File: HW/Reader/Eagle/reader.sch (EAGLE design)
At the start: 47 parts, among them Q4 BC817, U1 MCP16311, U2 ESP8266-12E

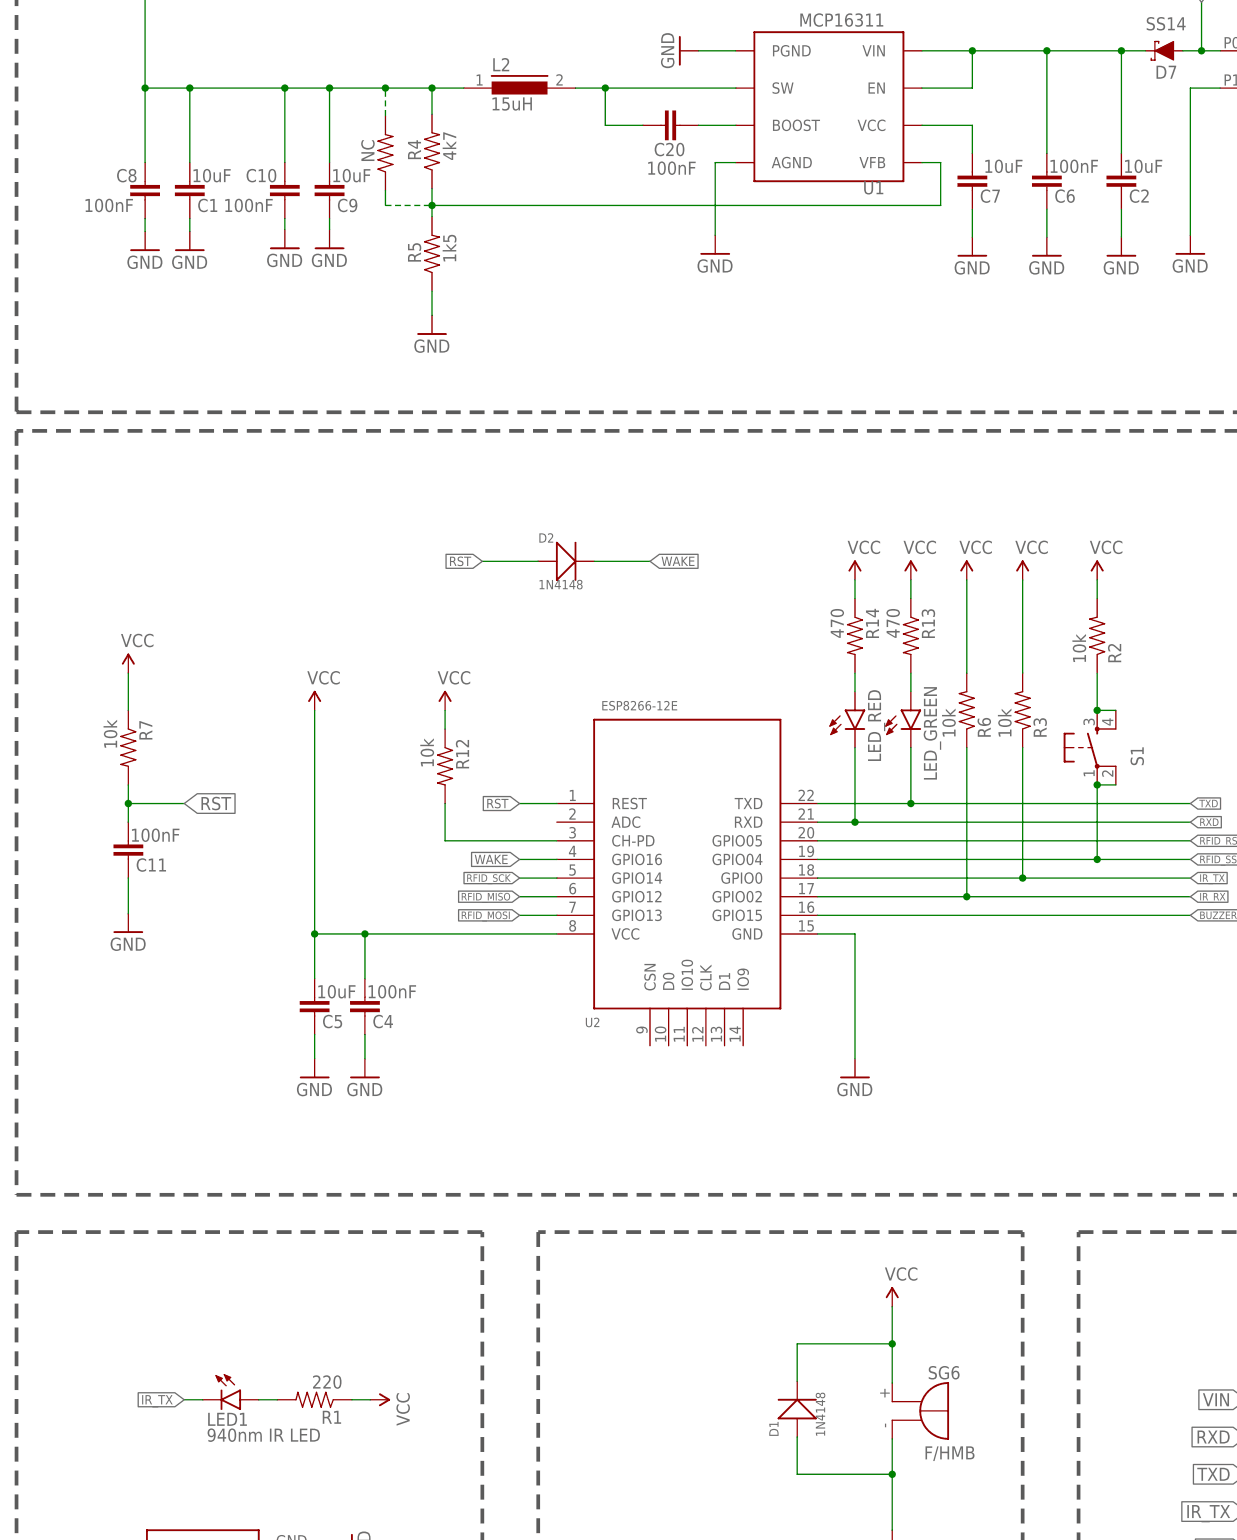
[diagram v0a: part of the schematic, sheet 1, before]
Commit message: Schematics are updated
Kickstart flasher PCB
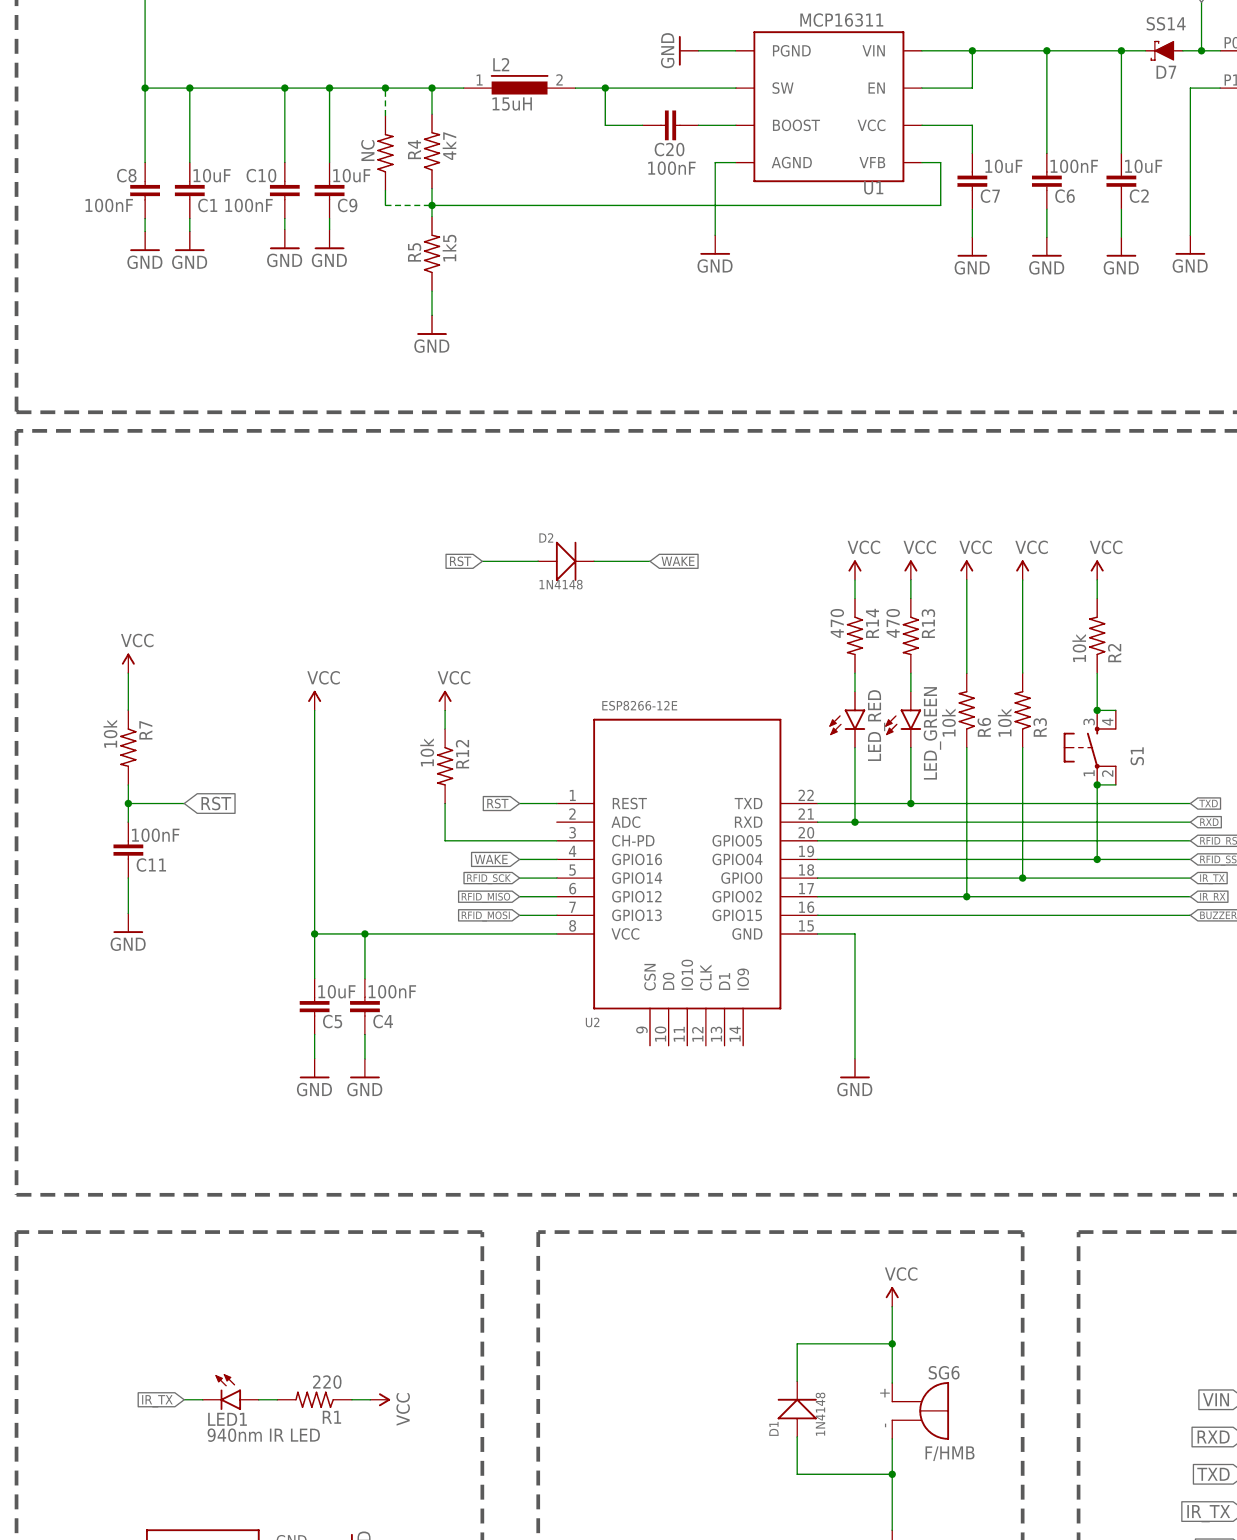
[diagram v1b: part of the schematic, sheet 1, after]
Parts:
- NC, R1, R12, R13, R14, R2, R3, R4, R5, R6, R7: device antduino:SPARKFUN_RESISTOR0805-RES -> rcl:R-US_M0805
- R10, R11: device adafruit:R-US_M0805 -> rcl:R-US_M0805
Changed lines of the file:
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@@
 <?xml version="1.0" encoding="utf-8"?>
 <!DOCTYPE eagle SYSTEM "eagle.dtd">
-<eagle version="9.6.0">
+<eagle version="9.6.1">
 <drawing>
 <settings>
@@
 <part name="GND17" library="supply1" deviceset="GND" device=""/>
 <part name="C12" library="rcl" library_urn="urn:adsk.eagle:library:334" deviceset="C-EU" device="C0805" package3d_urn="urn:adsk.eagle:package:23617/2" value="10uF"/>
-<part name="R1" library="antduino" deviceset="SPARKFUN_RESISTOR" device="0805-RES" value="220"/>
+<part name="R1" library="rcl" library_urn="urn:adsk.eagle:library:334" deviceset="R-US_" device="M0805" package3d_urn="urn:adsk.eagle:package:23556/2" value="220"/>
 <part name="GND3" library="supply1" library_urn="urn:adsk.eagle:library:371" deviceset="GND" device=""/>
 <part name="GND4" library="supply1" library_urn="urn:adsk.eagle:library:371" deviceset="GND" device=""/>
@@
 <part name="SUPPLY4" library="SparkFun-Aesthetics" deviceset="VCC" device=""/>
 <part name="Q4" library="dp_devices" deviceset="TRANSISTOR_BJT_NPN" device="-SOT-23-BCE" value="BC817"/>
-<part name="R10" library="adafruit" deviceset="R-US_" device="M0805" value="4k7"/>
-<part name="R11" library="adafruit" deviceset="R-US_" device="M0805" value="1K"/>
+<part name="R10" library="rcl" library_urn="urn:adsk.eagle:library:334" deviceset="R-US_" device="M0805" package3d_urn="urn:adsk.eagle:package:23556/2" value="4k7"/>
+<part name="R11" library="rcl" library_urn="urn:adsk.eagle:library:334" deviceset="R-US_" device="M0805" package3d_urn="urn:adsk.eagle:package:23556/2" value="1K"/>
 <part name="SUPPLY5" library="SparkFun-Aesthetics" deviceset="VCC" device=""/>
 <part name="SUPPLY6" library="SparkFun-Aesthetics" deviceset="VCC" device=""/>
@@
 <part name="GND18" library="supply1" deviceset="GND" device=""/>
 <part name="GND19" library="supply1" deviceset="GND" device=""/>
-<part name="R4" library="antduino" deviceset="SPARKFUN_RESISTOR" device="0805-RES" value="4k7"/>
-<part name="R5" library="antduino" deviceset="SPARKFUN_RESISTOR" device="0805-RES" value="1k5"/>
+<part name="R4" library="rcl" library_urn="urn:adsk.eagle:library:334" deviceset="R-US_" device="M0805" package3d_urn="urn:adsk.eagle:package:23556/2" value="4k7"/>
+<part name="R5" library="rcl" library_urn="urn:adsk.eagle:library:334" deviceset="R-US_" device="M0805" package3d_urn="urn:adsk.eagle:package:23556/2" value="1k5"/>
 <part name="GND20" library="supply1" deviceset="GND" device=""/>
-<part name="NC" library="antduino" deviceset="SPARKFUN_RESISTOR" device="0805-RES"/>
+<part name="NC" library="rcl" library_urn="urn:adsk.eagle:library:334" deviceset="R-US_" device="M0805" package3d_urn="urn:adsk.eagle:package:23556/2"/>
 <part name="SUPPLY7" library="SparkFun-Aesthetics" deviceset="VCC" device=""/>
 <part name="GND21" library="supply1" deviceset="GND" device=""/>
@@
 <part name="GND25" library="supply1" deviceset="GND" device=""/>
 <part name="M2" library="mfrc522-module" deviceset="RFID-RC522" device=""/>
-<part name="R12" library="antduino" deviceset="SPARKFUN_RESISTOR" device="0805-RES" value="10k"/>
+<part name="R12" library="rcl" library_urn="urn:adsk.eagle:library:334" deviceset="R-US_" device="M0805" package3d_urn="urn:adsk.eagle:package:23556/2" value="10k"/>
 <part name="SUPPLY3" library="SparkFun-Aesthetics" deviceset="VCC" device=""/>
 <part name="READER" library="frames" library_urn="urn:adsk.eagle:library:229" deviceset="FRAME_B_L" device=""/>
-<part name="R13" library="antduino" deviceset="SPARKFUN_RESISTOR" device="0805-RES" value="470"/>
-<part name="R14" library="antduino" deviceset="SPARKFUN_RESISTOR" device="0805-RES" value="470"/>
+<part name="R13" library="rcl" library_urn="urn:adsk.eagle:library:334" deviceset="R-US_" device="M0805" package3d_urn="urn:adsk.eagle:package:23556/2" value="470"/>
+<part name="R14" library="rcl" library_urn="urn:adsk.eagle:library:334" deviceset="R-US_" device="M0805" package3d_urn="urn:adsk.eagle:package:23556/2" value="470"/>
 <part name="SUPPLY9" library="SparkFun-Aesthetics" deviceset="VCC" device=""/>
 <part name="SUPPLY10" library="SparkFun-Aesthetics" deviceset="VCC" device=""/>
@@
 <part name="S1" library="SparkFun" deviceset="TAC_SWITCH" device="PTH" value="FLASH"/>
 <part name="U$1" library="Terminal Block Connector" deviceset="DBCONN-1X2" device=""/>
-<part name="R2" library="antduino" deviceset="SPARKFUN_RESISTOR" device="0805-RES" value="10k"/>
+<part name="R2" library="rcl" library_urn="urn:adsk.eagle:library:334" deviceset="R-US_" device="M0805" package3d_urn="urn:adsk.eagle:package:23556/2" value="10k"/>
 <part name="SUPPLY8" library="SparkFun-Aesthetics" deviceset="VCC" device=""/>
 <part name="TP1" library="testpad" library_urn="urn:adsk.eagle:library:385" deviceset="TP" device="TP20SQ" package3d_urn="urn:adsk.eagle:package:27980/1"/>
@@
 <part name="TP5" library="testpad" library_urn="urn:adsk.eagle:library:385" deviceset="TP" device="TP20SQ" package3d_urn="urn:adsk.eagle:package:27980/1"/>
 <part name="TP6" library="testpad" library_urn="urn:adsk.eagle:library:385" deviceset="TP" device="TP20SQ" package3d_urn="urn:adsk.eagle:package:27980/1"/>
-<part name="R3" library="antduino" deviceset="SPARKFUN_RESISTOR" device="0805-RES" value="10k"/>
+<part name="R3" library="rcl" library_urn="urn:adsk.eagle:library:334" deviceset="R-US_" device="M0805" package3d_urn="urn:adsk.eagle:package:23556/2" value="10k"/>
 <part name="SUPPLY11" library="SparkFun-Aesthetics" deviceset="VCC" device=""/>
-<part name="R6" library="antduino" deviceset="SPARKFUN_RESISTOR" device="0805-RES" value="10k"/>
+<part name="R6" library="rcl" library_urn="urn:adsk.eagle:library:334" deviceset="R-US_" device="M0805" package3d_urn="urn:adsk.eagle:package:23556/2" value="10k"/>
 <part name="SUPPLY12" library="SparkFun-Aesthetics" deviceset="VCC" device=""/>
-<part name="R7" library="antduino" deviceset="SPARKFUN_RESISTOR" device="0805-RES" value="10k"/>
+<part name="R7" library="rcl" library_urn="urn:adsk.eagle:library:334" deviceset="R-US_" device="M0805" package3d_urn="urn:adsk.eagle:package:23556/2" value="10k"/>
 <part name="C11" library="rcl" library_urn="urn:adsk.eagle:library:334" deviceset="C-EU" device="C0805" package3d_urn="urn:adsk.eagle:package:23617/2" value="100nF"/>
 <part name="GND1" library="supply1" deviceset="GND" device=""/>
